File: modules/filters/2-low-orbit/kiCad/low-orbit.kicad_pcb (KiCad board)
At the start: 2 copper layers, 81 x 111 mm, 94 parts, among them J1 IN, J2 CV_INPUT_1, J3 CV_INPUT_2, J4 PWR, J5 FILTER_OUT, Q1 BC548, U1 TL074, U2 TL074

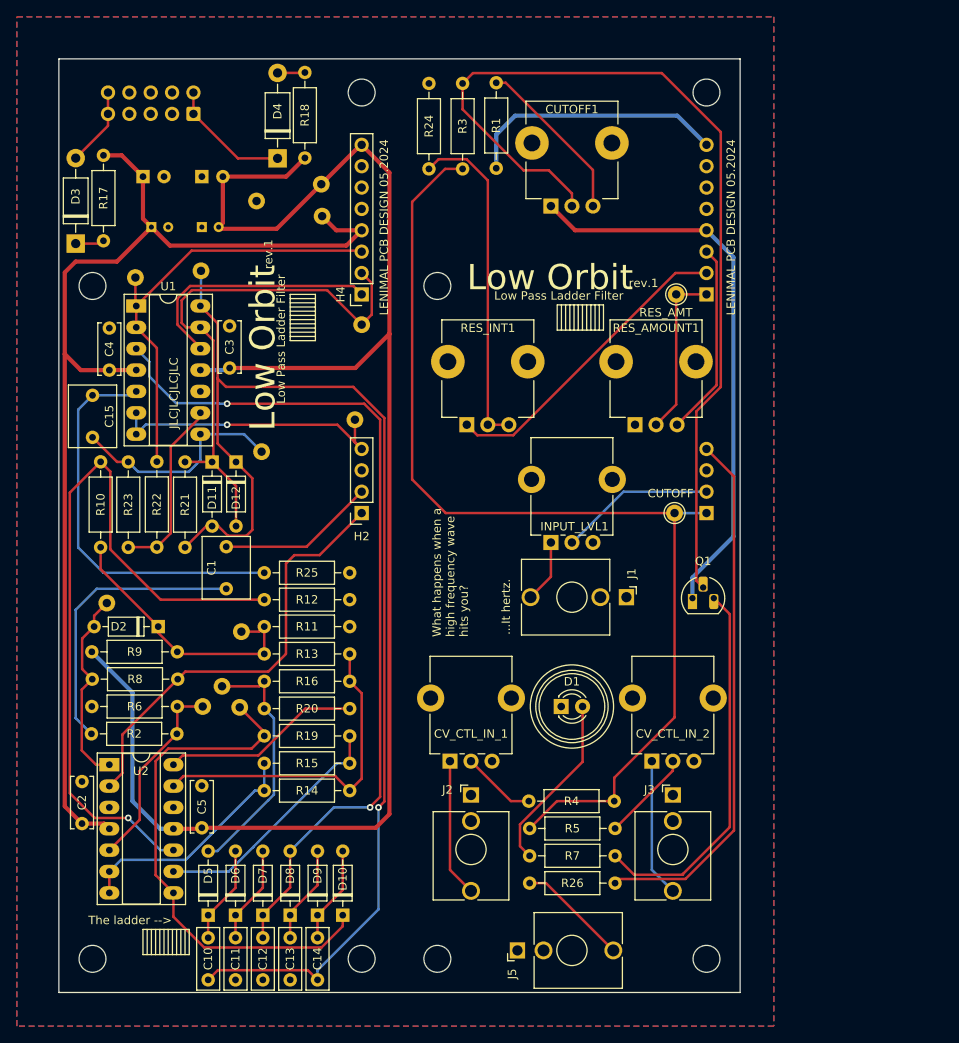
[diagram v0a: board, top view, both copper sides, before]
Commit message: update components, PCB 3320 and design
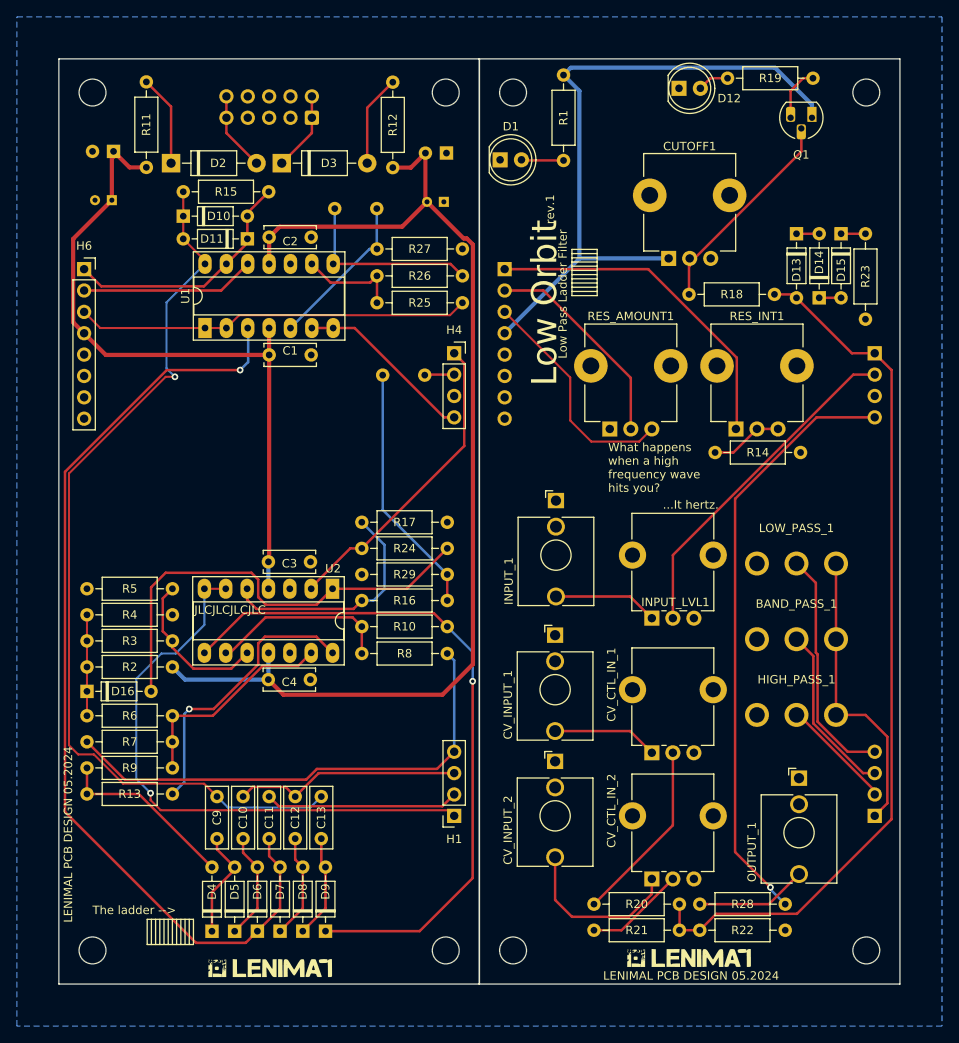
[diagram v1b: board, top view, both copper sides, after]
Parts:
- removed J2: CV_INPUT_1, Synth:Jack_3.5mm_QingPu_WQP-PJ398SM_Vertical_CircularHoles
- removed J3: CV_INPUT_2, Synth:Jack_3.5mm_QingPu_WQP-PJ398SM_Vertical_CircularHoles
- removed J4: PWR, Synth:IDC-Header_2x05_P2.54mm_Vertical
- removed J5: FILTER_OUT, Synth:Jack_3.5mm_QingPu_WQP-PJ398SM_Vertical_CircularHoles
- removed TP1: INPUT, Connector_Pin:Pin_D1.0mm_L10.0mm
- removed TP10: RES_AMT, Connector_Pin:Pin_D1.0mm_L10.0mm
- removed TP11: PRE_OUT, Connector_Pin:Pin_D1.0mm_L10.0mm
- removed TP12: OUT, Connector_Pin:Pin_D1.0mm_L10.0mm
- removed TP13: +12V, Connector_Pin:Pin_D1.0mm_L10.0mm
- removed TP14: -12V, Connector_Pin:Pin_D1.0mm_L10.0mm
- removed TP15: GND, Connector_Pin:Pin_D1.0mm_L10.0mm
- removed TP2: CUTOFF, Connector_Pin:Pin_D1.0mm_L10.0mm
- removed TP3: CUTOFF_BUFF, Connector_Pin:Pin_D1.0mm_L10.0mm
- removed TP4: CUTOFF_REF, Connector_Pin:Pin_D1.0mm_L10.0mm
- removed TP5: RES_FEEDBACK, Connector_Pin:Pin_D1.0mm_L10.0mm
- removed TP6: POS_INPUT, Connector_Pin:Pin_D1.0mm_L10.0mm
- removed TP7: NEG_INPUT, Connector_Pin:Pin_D1.0mm_L10.0mm
- removed TP8: RES_INTENSITY, Connector_Pin:Pin_D1.0mm_L10.0mm
- removed TP9: FILTER_OUT, Connector_Pin:Pin_D1.0mm_L10.0mm
- added BAND_PASS_1: BAND_PASS, Synth:SW_default, F.Cu at (137.7, 119.0)
- added CV_INPUT_1: CV_INPUT_1, Synth:Jack_3.5mm_QingPu_WQP-PJ398SM_Vertical_CircularHoles, F.Cu at (109.0, 125.0)
- added CV_INPUT_2: CV_INPUT_2, Synth:Jack_3.5mm_QingPu_WQP-PJ398SM_Vertical_CircularHoles, F.Cu at (109.0, 140.0)
- added D13: 1N4148, Synth:D_DO-35_SOD27_P7.62mm_Horizontal, F.Cu at (137.7, 70.8)
- added D14: 1N4148, Synth:D_DO-35_SOD27_P7.62mm_Horizontal, F.Cu at (140.4, 78.4)
- added D15: 1N4148, Synth:D_DO-35_SOD27_P7.62mm_Horizontal, F.Cu at (143.0, 70.8)
- added D16: 1N4148, Synth:D_DO-35_SOD27_P7.62mm_Horizontal, F.Cu at (53.3, 125.2)
- added G***: LOGO, Synth:lenimal_logo_full, F.Cu at (125.0, 156.9)
- added G***: LOGO, Synth:lenimal_logo_full, F.Cu at (75.2, 158.1)
- added G***: LOGO, Synth:lenimal_logo_full, B.Cu at (75.0, 158.1)
- added H13: MountingHole, MountingHole:MountingHole_3.2mm_M3, F.Cu at (146.0, 54.0)
- added H14: MountingHole, MountingHole:MountingHole_3.2mm_M3, F.Cu at (146.0, 156.0)
- added HIGH_PASS_1: HIGH_PASS, Synth:SW_default, F.Cu at (137.7, 128.0)
- added INPUT_1: IN, Synth:Jack_3.5mm_QingPu_WQP-PJ398SM_Vertical_CircularHoles, F.Cu at (109.1, 109.0)
- added LOW_PASS_1: LOW_PASS, Synth:SW_default, F.Cu at (137.7, 110.0)
- added OUTPUT_1: FILTER_OUT, Synth:Jack_3.5mm_QingPu_WQP-PJ398SM_Vertical_CircularHoles, F.Cu at (138.0, 142.0)
- added R27: 100K, Synth:R_Default (DIN0207), F.Cu at (98.0, 72.6)
- added R28: 1K, Synth:R_Default (DIN0207), F.Cu at (126.2, 150.5)
- added R29: 100K, Synth:R_Default (DIN0207), F.Cu at (96.2, 111.3)
- C1: value C_1uF (MKS) -> 0.1uF; footprint Synth:C_RECT_MKT_1uF -> Capacitor_THT:C_Disc_D6.0mm_W2.5mm_P5.00mm
- C14: value 1nF [2,5%] -> 1uF; footprint Synth:C_RECT_WIMA_0.1uF -> Synth:C_RECT_MKT_1uF; moved to B.Cu
- C15: moved to B.Cu
- C5: value 0.1uF -> 47uF; footprint Capacitor_THT:C_Disc_D6.0mm_W2.5mm_P5.00mm -> Capacitor_THT:CP_Radial_D6.3mm_P2.50mm; moved to B.Cu
- C7: value 47uF -> 0.1uF; footprint Capacitor_THT:CP_Radial_D6.3mm_P2.50mm -> Capacitor_THT:CP_Radial_D4.0mm_P2.00mm
- C9: value 0.1uF -> 1nF [2,5%]; footprint Capacitor_THT:CP_Radial_D4.0mm_P2.00mm -> Synth:C_RECT_WIMA_0.1uF; moved to F.Cu
- D1: footprint LED_THT:LED_D3.0mm -> Synth:LED_D5.0mm (center Aligned)
- D12: value 1N4148 -> LED; footprint Synth:D_DO-35_SOD27_P7.62mm_Horizontal -> Synth:LED_D5.0mm (center Aligned)
- D2: value 1N4148 -> 1N5819; footprint Synth:D_DO-35_SOD27_P7.62mm_Horizontal -> Synth:D_DO-41_SOD81_P10.16mm_Horizontal
- D4: value 1N5819 -> 1N4148; footprint Synth:D_DO-41_SOD81_P10.16mm_Horizontal -> Synth:D_DO-35_SOD27_P7.62mm_Horizontal
- H1: value TOP_4_SGL -> PinHeader_01x04; footprint Synth:PinHeader_1x04_P2.54mm_Vertical -> Synth:PinSocket_1x04_P2.54mm_Vertical; moved to F.Cu
- H2: value BTM_4_SGL -> PinSocket_01x04; footprint Synth:PinSocket_1x04_P2.54mm_Vertical -> Synth:PinHeader_1x04_P2.54mm_Vertical; moved to B.Cu
- H4: value BTM_8_SGL -> BTM_4_SGL; footprint Synth:PinSocket_1x08_P2.54mm_Vertical -> Synth:PinSocket_1x04_P2.54mm_Vertical
- H5: value MountingHole -> TOP_4_SGL; footprint MountingHole:MountingHole_3.2mm_M3 -> Synth:PinHeader_1x04_P2.54mm_Vertical; moved to B.Cu
- H6: value MountingHole -> BTM_8_SGL; footprint MountingHole:MountingHole_3.2mm_M3 -> Synth:PinSocket_1x08_P2.54mm_Vertical
- J1: value IN -> PWR; footprint Synth:Jack_3.5mm_QingPu_WQP-PJ398SM_Vertical_CircularHoles -> Synth:IDC-Header_2x05_P2.54mm_Vertical; moved to B.Cu
- R1: value 27K [1%] -> 470
- R11: value 27K [1%] -> 10R
- R12: value 33K [1%] -> 10R
- R13: value 33K [1%] -> 2K
- R14: value 33K [1%] -> 1K [1%]
- R15: value 33K [1%] -> 100K
- R16: value 33K [1%] -> 33K
- R17: value 10 -> 680R
- R18: value 10 -> 100K
- R19: value 33K [1%] -> 470
- R2: value 100K [1%] -> 100K
- R20: value 2K [1%] -> 47K [1%]
- R21: value 100K [1%] -> 47K [1%]
- R22: value 1K [1%] -> 47K [1%]
- R23: value 33K [1%] -> 1K
- R24: value 1K [1%] -> 14K [1%]
- R25: value 100K [1%] -> 1K
- R26: value 1K [1%] -> 33K
- R3, R9: value 100K [1%] -> 33K [1%]
- R4: value 68K [1%] -> 27K
- R5: value 68K [1%] -> 33K [1%]
- R6: value 2K [1%] -> 33K [1%]
- R7: value 470 -> 33K [1%]
- R8: value 14K [1%] -> 33K [1%]
- moved R19 101.8 mm to (139.6, 52.3), turned to 180 degrees
- moved R23 95.2 mm to (145.9, 70.8), turned to -90 degrees
- moved D4 92.3 mm to (68.2, 153.7)
- moved R22 85.3 mm to (126.2, 153.6), turned to 0 degrees
- moved D10 85.2 mm to (64.8, 68.7), turned to 0 degrees
- moved H6 82.0 mm to (53.0, 75.0)
- moved C5 76.1 mm to (56.5, 61.0), turned to 180 degrees
- moved C2 74.9 mm to (80.0, 71.2), turned to 180 degrees
- moved R26 74.4 mm to (87.8, 75.8)
- moved R21 74.3 mm to (123.8, 153.6), turned to 180 degrees
- moved C14 73.0 mm to (93.5, 87.6), turned to 180 degrees
- moved H2 70.8 mm to (147.0, 140.0), turned to 0 degrees
- moved D12 69.9 mm to (125.0, 53.5), turned to 0 degrees
- moved R15 68.6 mm to (64.8, 65.8)
- moved C9 67.7 mm to (68.8, 137.7), turned to -90 degrees
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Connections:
- net Net-(H3C-Pin_3) renamed /resonance/input
- C1 pad 1: Net-(H2B-Pin_2) -> +12V
- C1 pad 2: Net-(C1-Pad2) -> GNDREF
- C10 pad 1: Net-(D11-A) -> Net-(H1C-Pin_3)
- C11 pad 1: GNDREF -> Net-(H1B-Pin_2)
- C12 pad 1: GNDREF -> Net-(H1C-Pin_3)
- C13 pad 1: GNDREF -> /resonance/output
- C14 pad 1: Net-(D11-A) -> Net-(H4B-Pin_2)
- C14 pad 2: Net-(D10-A) -> Net-(C14-Pad2)
- C2 pad 1: +12V -> GNDREF
- C2 pad 2: GNDREF -> -12V
- C3 pad 1: GNDREF -> +12V
- C3 pad 2: -12V -> GNDREF
- C4 pad 1: +12V -> GNDREF
- C4 pad 2: GNDREF -> -12V
- C5 pad 1: GNDREF -> +12V
- C5 pad 2: -12V -> GNDREF
- C6 pad 1: +12V -> GNDREF
- C6 pad 2: GNDREF -> -12V
- C7 pad 1: GNDREF -> +12V
- C7 pad 2: -12V -> GNDREF
- C8 pad 1: +12V -> GNDREF
- C8 pad 2: GNDREF -> -12V
- C9 pad 1: GNDREF -> /resonance/output
- C9 pad 2: -12V -> Net-(D4-K)
- CUTOFF1 pad 3: Net-(CUTOFF1-Pad3) -> GNDREF
- D10 pad 1: Net-(D10-K) -> /resonance/output
- D11 pad 1: Net-(D11-K) -> Net-(D10-A)
- D11 pad 2: Net-(D11-A) -> /resonance/output
- D12 pad 1: Net-(D11-A) -> GNDREF
- D12 pad 2: Net-(D11-K) -> Net-(D12-A)
- D5 pad 2: Net-(D5-A) -> Net-(D4-K)
- D9 pad 1: Net-(D10-A) -> Net-(D9-K)
- H1 pad 1: Net-(H1A-Pin_1) -> /input/output
- H1 pad 3: GNDREF -> Net-(H1C-Pin_3)
- H2 pad 1: Net-(H2A-Pin_1) -> Net-(BAND_PASS_1-C)
- H2 pad 3: GNDREF -> Net-(BAND_PASS_1-B)
- H3 pad 8: -12V -> GNDREF
- H4 pad 1: Net-(H4A-Pin_3) -> Net-(H4A-Pin_1)
- H4 pad 2: Net-(D11-K) -> Net-(H4B-Pin_2)
- H4 pad 3: Net-(H4C-Pin_3) -> GNDREF
- H4 pad 4: +12V -> Net-(H4D-Pin_4)
- INPUT_LVL1 pad 1: Net-(INPUT_LVL1-Pad1) -> Net-(INPUT_1-PadT)
- INPUT_LVL1 pad 2: Net-(H1B-Pin_2) -> Net-(H5B-Pin_2)
- R1 pad 1: Net-(CUTOFF1-Pad3) -> +12V
- R1 pad 2: -12V -> Net-(D1-A)
- R10 pad 1: Net-(U2C-+) -> Net-(D9-K)
- R10 pad 2: Net-(D2-K) -> Net-(U2C--)
- R11 pad 1: GNDREF -> +12V
- R12 pad 1: GNDREF -> -12V
- R12 pad 2: Net-(U2C-+) -> Net-(D3-A)
- R13 pad 1: Net-(D2-K) -> Net-(R13-Pad1)
- R13 pad 2: Net-(U2D--) -> Net-(D4-A)
- R14 pad 1: Net-(U2B--) -> Net-(R14-Pad1)
- R14 pad 2: Net-(U2D--) -> GNDREF
- R15 pad 1: Net-(U2B--) -> /resonance/output
- R15 pad 2: Net-(U2C--) -> Net-(D10-A)
- R16 pad 1: Net-(U2D--) -> Net-(U2B-+)
- R16 pad 2: Net-(D5-A) -> Net-(C14-Pad2)
- R17 pad 1: +12V -> GNDREF
- R17 pad 2: Net-(D3-K) -> Net-(U2B-+)
- R18 pad 1: -12V -> Net-(D13-A)
- R18 pad 2: Net-(D4-A) -> Net-(Q1-B)
- R19 pad 1: Net-(D10-K) -> Net-(Q1-E)
- R19 pad 2: Net-(U2C--) -> Net-(D12-A)
- R2 pad 1: Net-(U2B-+) -> /cv-input/cv_out
- R2 pad 2: Net-(C1-Pad2) -> -12V
- R20 pad 1: Net-(R20-Pad1) -> Net-(D13-A)
- R20 pad 2: Net-(D5-A) -> Net-(CV_CTL_IN_1-Pad2)
- R21 pad 1: Net-(D11-A) -> Net-(D13-A)
- R21 pad 2: Net-(D11-K) -> Net-(CV_CTL_IN_2-Pad2)
- R22 pad 1: Net-(H4C-Pin_3) -> Net-(D13-A)
- R22 pad 2: Net-(U1C--) -> GNDREF
- R23 pad 1: Net-(U1C--) -> Net-(D15-K)
- R23 pad 2: Net-(C15-Pad1) -> GNDREF
- R24 pad 1: Net-(R24-Pad1) -> Net-(D16-A)
- R24 pad 2: GNDREF -> Net-(H4A-Pin_1)
- R25 pad 1: GNDREF -> /output/input
- R25 pad 2: Net-(U1B-+) -> Net-(U1C--)
- R26 pad 1: Net-(J5-PadT) -> Net-(U1C--)
- R26 pad 2: Net-(H1D-Pin_4) -> Net-(C15-Pad1)
- R3 pad 1: Net-(H1A-Pin_1) -> Net-(U2C-+)
- R3 pad 2: Net-(Q1-B) -> /cv-input/cv_out
- R4 pad 1: Net-(H1A-Pin_1) -> GNDREF
- R4 pad 2: Net-(CV_CTL_IN_1-Pad2) -> /cv-input/cv_out
- R5 pad 1: Net-(H1A-Pin_1) -> GNDREF
- R5 pad 2: Net-(CV_CTL_IN_2-Pad2) -> Net-(U2C-+)
- R6 pad 1: GNDREF -> /cv-input/cv_out
- R6 pad 2: Net-(U2B-+) -> Net-(U2D--)
- R7 pad 1: Net-(Q1-E) -> Net-(H1D-Pin_4)
- R7 pad 2: Net-(D1-A) -> Net-(U2D--)
- R8 pad 1: Net-(D2-A) -> Net-(H1D-Pin_4)
- R8 pad 2: Net-(H2A-Pin_1) -> Net-(U2C--)
- R9 pad 1: Net-(D2-K) -> Net-(U2D--)
- R9 pad 2: -12V -> Net-(D4-A)
- RES_AMOUNT1 pad 2: Net-(H3A-Pin_1) -> Net-(H3B-Pin_2)
- RES_INT1 pad 1: Net-(H3B-Pin_2) -> Net-(H3A-Pin_1)
- RES_INT1 pad 2: Net-(R24-Pad1) -> Net-(R14-Pad1)
- RES_INT1 pad 3: Net-(R24-Pad1) -> Net-(R14-Pad1)
- U1 pad 1: Net-(H4C-Pin_3) -> /output/input
- U1 pad 12: Net-(H4A-Pin_3) -> Net-(H6B-Pin_2)
- U1 pad 13: Net-(D11-K) -> Net-(D10-A)
- U1 pad 14: Net-(D11-A) -> /resonance/output
- U1 pad 2: Net-(H4C-Pin_3) -> /output/input
- U1 pad 3: Net-(D7-K) -> Net-(D6-K)
- U1 pad 6: Net-(H2D-Pin_4) -> Net-(H4D-Pin_4)
- U1 pad 7: Net-(H2D-Pin_4) -> Net-(H4D-Pin_4)
- U2 pad 1: Net-(D2-A) -> Net-(D16-A)
- U2 pad 14: Net-(R20-Pad1) -> Net-(R13-Pad1)
- U2 pad 2: Net-(H2A-Pin_1) -> Net-(H4A-Pin_1)
- U2 pad 6: Net-(U2B--) -> /input/output
- U2 pad 7: Net-(U2B--) -> /input/output
- U2 pad 8: Net-(D10-K) -> Net-(D9-K)
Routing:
- net Net-(D11-A): track 149.2 -> 0.00 mm, vias 1 -> 0
- net Net-(H1A-Pin_1): track 125.9 -> 0.00 mm
- net /resonance/output: track 0.00 -> 108.6 mm, vias 0 -> 1
- net Net-(D13-A): track 0.00 -> 104.8 mm
- net Net-(D6-K): track 11.7 -> 114.2 mm, vias 0 -> 1
- net -12V: track 227.1 -> 133.4 mm
- net Net-(D7-K): track 103.4 -> 12.5 mm, vias 2 -> 0
- net Net-(Q1-B): track 111.5 -> 25.6 mm
- net Net-(D9-K): track 0.00 -> 82.8 mm, vias 0 -> 1
- net Net-(H5D-Pin_4): track 0.00 -> 71.3 mm, vias 0 -> 1
- net /input/output: track 0.00 -> 70.9 mm, vias 0 -> 1
- net Net-(U2C-+): track 87.7 -> 18.6 mm, vias 1 -> 0
- net Net-(D11-K): track 64.6 -> 0.00 mm
- net Net-(D10-K): track 62.2 -> 0.00 mm
- net Net-(D16-A): track 0.00 -> 53.9 mm
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- removed copper zone on F.Cu, net (none)
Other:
- board size 81 x 111 mm -> 100 x 110 mm
- board text added: "TODO: SHIFT BY 1 MM FOR V SCORE"
- board text removed: "+12V"
- board text removed: "-12V"
- board text removed: "CUTOFF"
- board text removed: "CUTOFF_BFR"
- board text removed: "CUTOFF_PRE"
- board text removed: "FILTER_OUT"
- board text removed: "GND"
- board text removed: "INPUT"
- board text removed: "NEG_INPUT"
- board text removed: "OUTPUT"
- board text removed: "POS_INPUT"
- board text removed: "PRE_OUT"
- board text removed: "RES_AMT"
- board text removed: "RES_FEEDBACK"
- board text removed: "RES_INTENSE"
